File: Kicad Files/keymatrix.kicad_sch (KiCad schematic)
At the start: 143 parts, among them SW1 GRAVE, SW10 9, SW11 0, SW12 -, SW13 +, SW14 BSPC, SW15 DEL, SW16 TAB, SW17 Q, SW18 W, SW19 E, SW2 1, SW20 R, SW21 T, SW22 Y, SW23 U, SW24 I, SW25 O, SW26 P, SW27 [, SW28 ], SW29 SPLIT_BS, SW3 2, SW30 PGUP, SW31 CAPS, SW32 A, SW33 S, SW34 D, SW35 F, SW36 G, SW37 H, SW38 J, SW39 K, SW4 3, SW40 L, SW41 COLON, SW42 QUOTE, SW43 BSLS, SW44 ENTER, SW45 PGDN, SW46 LSFT, SW47 Z, SW48 X, SW49 C, SW5 4, SW50 V, SW51 B, SW52 N, SW53 M, SW54 COMMA, SW55 DOT, SW56 SLSH, SW57 RSFT, SW58 UP, SW59 END, SW6 5, SW60 LCTL, SW61 LGUI, SW62 LALT, SW63 6.25U SPC, SW64 RALT, SW65 RCTL, SW66 LEFT, SW67 DOWN, SW68 RIGHT, SW69 1.5U LCTL, SW7 6, SW70 1U LGUI, SW71 1.5U LALT, SW72 7U SPC, SW73 1.5U MO1, SW74 SPLIT_BSLS, SW75 STEPPED CAPS, SW8 7, SW9 8

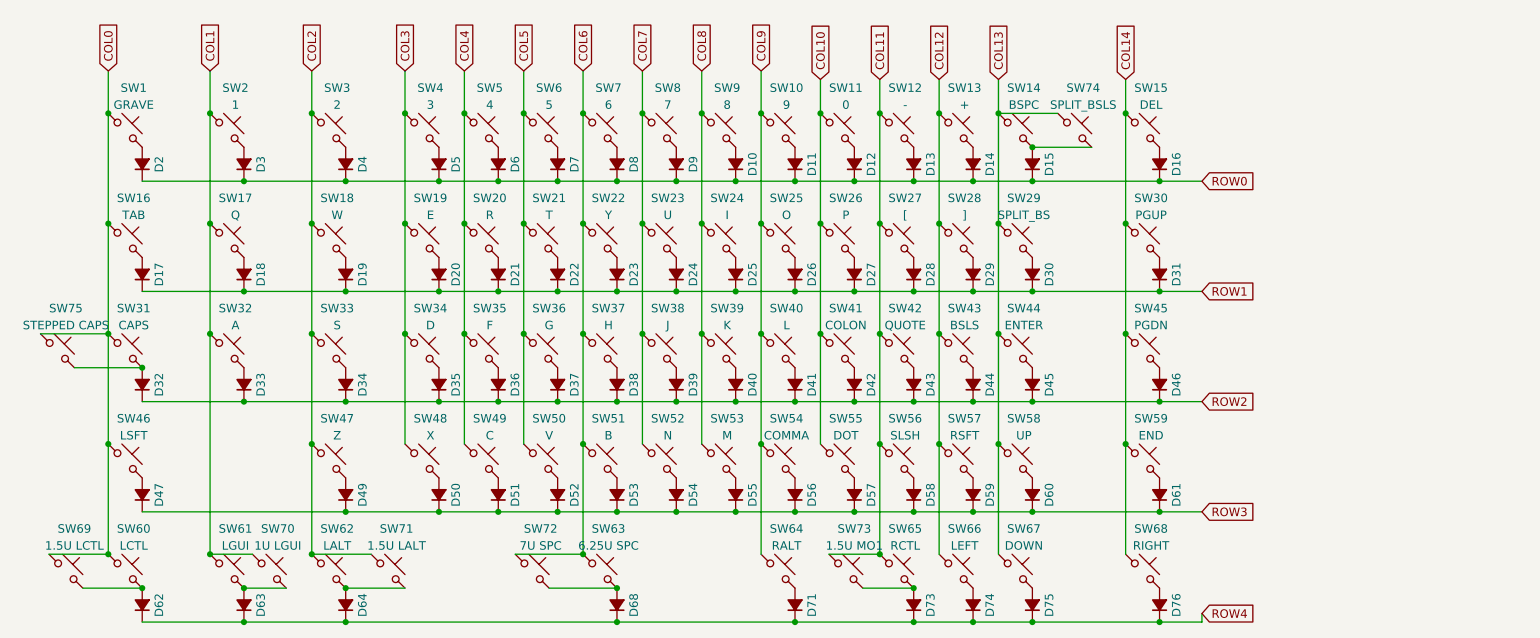
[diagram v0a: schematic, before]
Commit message: Edited BackSplit
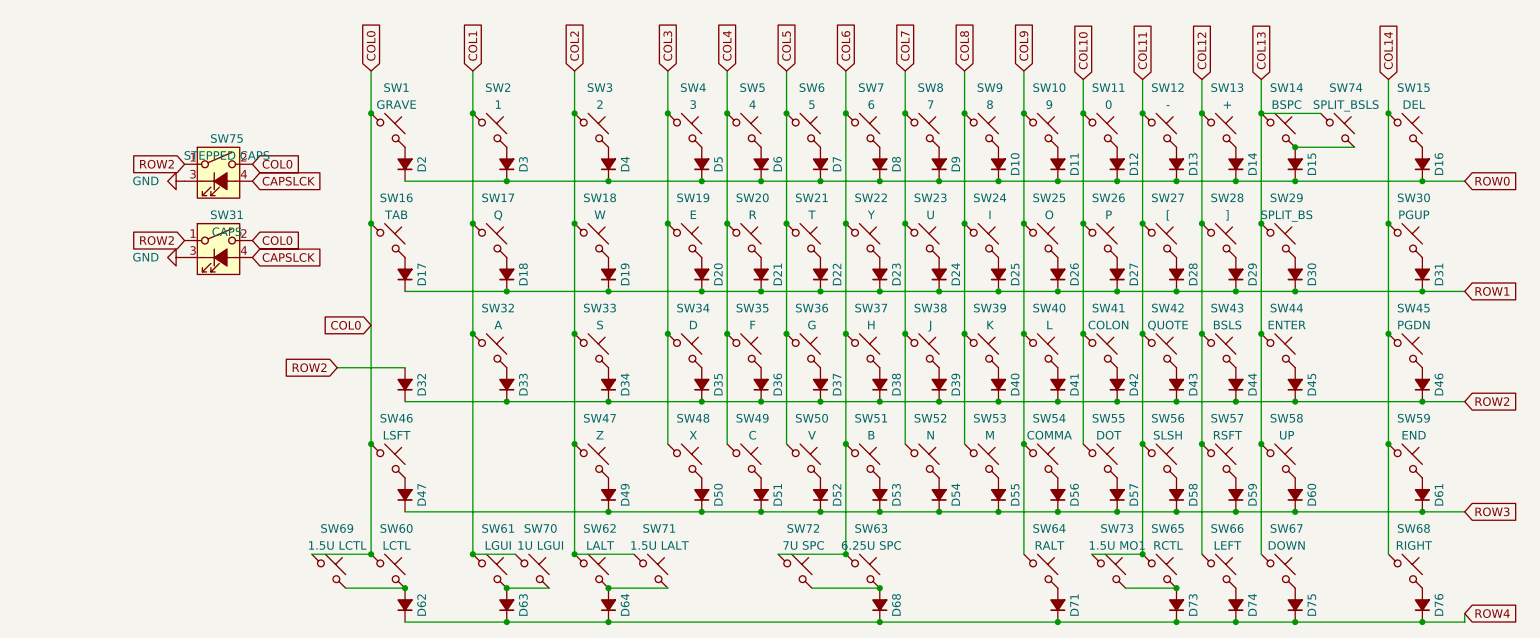
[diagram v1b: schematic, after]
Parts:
- SW1, SW10, SW11, SW12, SW13, SW15, SW17, SW18, SW19, SW2, SW20, SW21, SW22, SW23, SW24, SW25, SW26, SW27, SW28, SW29, SW3, SW30, SW32, SW33, SW34, SW35, SW36, SW37, SW38, SW39, SW4, SW40, SW41, SW42, SW45, SW47, SW48, SW49, SW5, SW50, SW51, SW52, SW53, SW54, SW55, SW56, SW58, SW59, SW6, SW66, SW67, SW68, SW7, SW70, SW74, SW8, SW9: footprint PCM_Switch_Keyboard_Cherry_MX:SW_Cherry_MX_PCB_1.00u_valueprint -> CherryMX_PCB:CherryMX_1.00u_PCB
- SW14: footprint PCM_Switch_Keyboard_Cherry_MX:SW_Cherry_MX_PCB_2.00u_valueprint -> CherryMX_PCB_StabWireBottom:CherryMX_2.00u_PCB_StabWireBottom
- SW16, SW43, SW69, SW71, SW73: footprint PCM_Switch_Keyboard_Cherry_MX:SW_Cherry_MX_PCB_1.50u_valueprint -> CherryMX_PCB:CherryMX_1.50u_PCB
- SW31: footprint PCM_Switch_Keyboard_Cherry_MX:SW_Cherry_MX_PCB_1.75u_valueprint -> CherryMX_PCB:CherryMX_1.75u_PCB; symbol Switch:SW_Push_45deg -> Switch:SW_SPST_LED
- SW44, SW46: footprint PCM_Switch_Keyboard_Cherry_MX:SW_Cherry_MX_PCB_2.25u_valueprint -> CherryMX_PCB_StabWireBottom:CherryMX_2.25u_PCB_StabWireBottom
- SW57: footprint PCM_Switch_Keyboard_Cherry_MX:SW_Cherry_MX_PCB_1.75u_valueprint -> CherryMX_PCB:CherryMX_1.75u_PCB
- SW60, SW61, SW62, SW64, SW65: footprint PCM_Switch_Keyboard_Cherry_MX:SW_Cherry_MX_PCB_1.25u_valueprint -> CherryMX_PCB:CherryMX_1.25u_PCB
- SW63: footprint PCM_Switch_Keyboard_Cherry_MX:SW_Cherry_MX_PCB_6.25u -> CherryMX_PCB_StabWireTop:CherryMX_6.25u_PCB_StabWireTop
- SW72: footprint PCM_Switch_Keyboard_Cherry_MX:SW_Cherry_MX_PCB_7.00u -> CherryMX_PCB_StabWireTop:CherryMX_7.00u_PCB_StabWireTop
- SW75: footprint PCM_Switch_Keyboard_Cherry_MX:SW_Cherry_MX_PCB_1.25u_valueprint -> CherryMX_PCB:CherryMX_1.25u_PCB; symbol Switch:SW_Push_45deg -> Switch:SW_SPST_LED
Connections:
- net ROW2: now also D32.2 (A), SW31.1, SW75.1
- new net CAPSLCK: SW31.4 (A), SW75.4 (A)
- new net GND: SW31.3 (K), SW75.3 (K)
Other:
- moved on the sheet: D10, D11, D12, D13, D14, D15, D16, D17, D18, D19, D2, D20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
